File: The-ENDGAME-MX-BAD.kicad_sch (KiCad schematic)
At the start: 76 parts, among them J2 Conn_01x02_Female, SW1 SW_Push, SW10 SW_Push, SW11 SW_Push, SW12 SW_Push, SW13 SW_Push, SW14 SW_Push, SW15 SW_Push, SW16 SW_Push, SW17 SW_Push, SW18 SW_Push, SW19 SW_Push, SW2 SW_Push, SW20 SW_Push, SW21 SW_Push, SW22 SW_Push, SW23 SW_Push, SW24 SW_Push, SW25 SW_Push, SW26 SW_Push, SW27 SW_Push, SW28 SW_Push, SW29 SW_Push, SW3 SW_Push, SW30 SW_Push, SW31 SW_Push, SW32 SW_Push, SW33 SW_Push, SW34 SW_Push, SW35 SW_Push, SW36 SW_Push, SW4 SW_Push, SW5 SW_Push, SW6 SW_Push, SW7 SW_Push, SW8 SW_Push, SW9 SW_Push, U1 ProMicro-kbd-34key

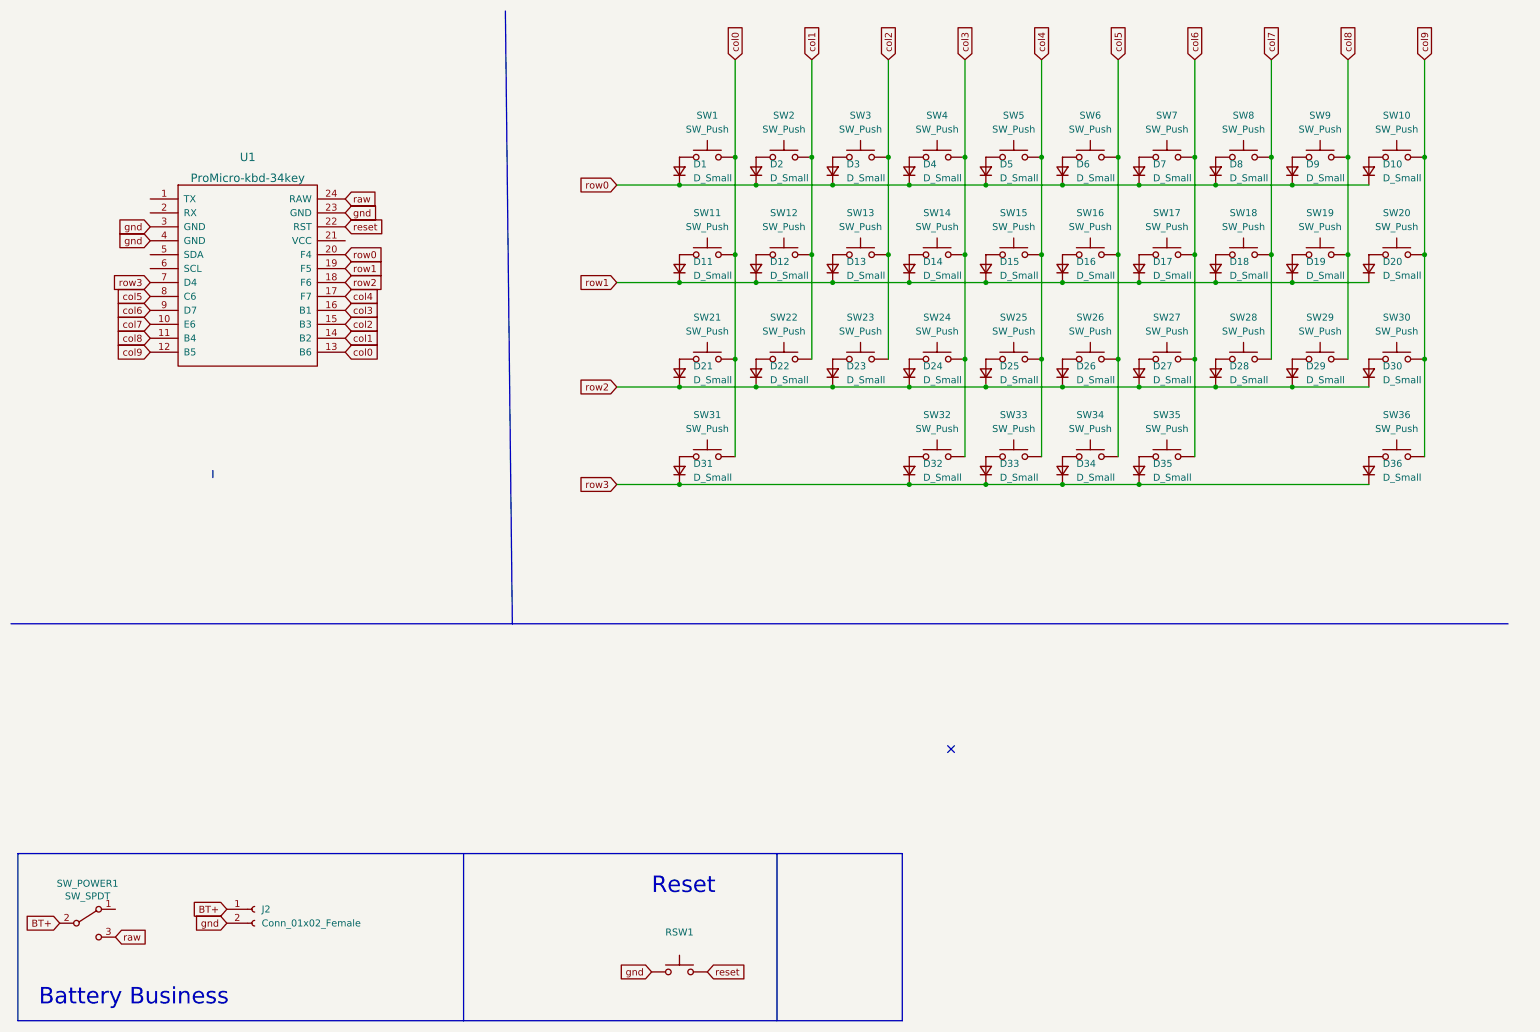
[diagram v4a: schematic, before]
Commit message: ja ja push den scheis
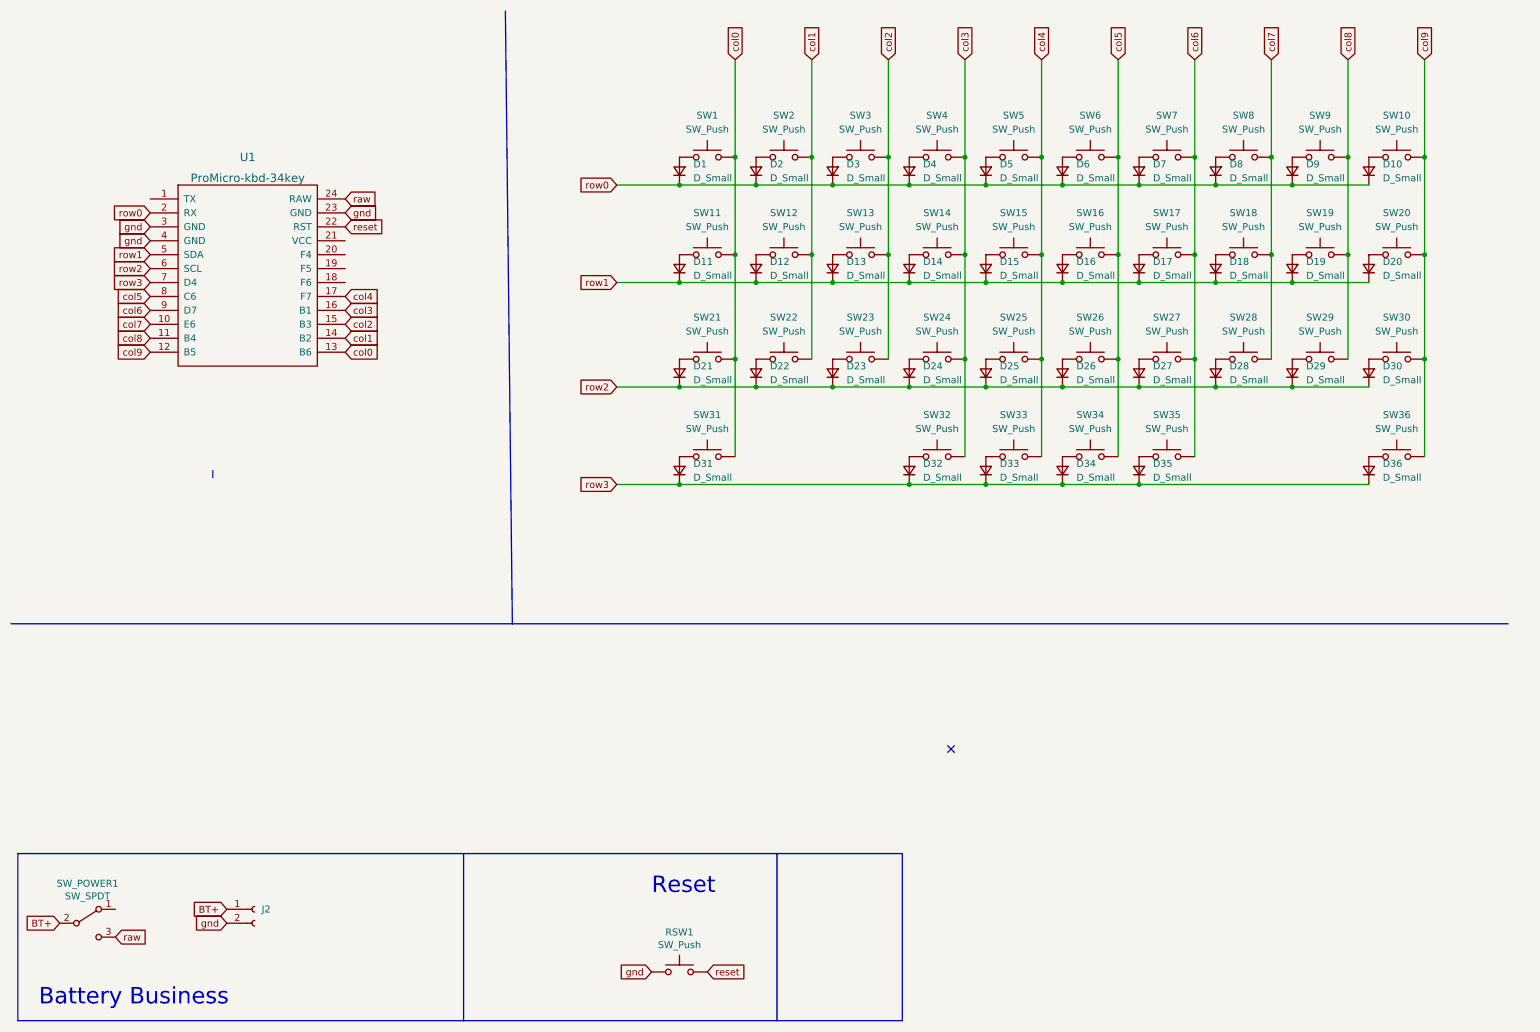
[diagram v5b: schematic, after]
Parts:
- J2: value Conn_01x02_Female -> (none); footprint Connector_JST:JST_SH_BM02B-SRSS-TB_1x02-1MP_P1.00mm_Vertical -> (none)
- RSW1: value (none) -> SW_Push; footprint (none) -> Button_Switch_SMD:SW_SPST_TL3342
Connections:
- net row0: now also U1.2 (RX); no longer U1.20 (F4)
- net row1: now also U1.5 (SDA); no longer U1.19 (F5)
- net row2: now also U1.6 (SCL); no longer U1.18 (F6)
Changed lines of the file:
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@@
     )
   )
-  (global_label "row1" (shape input) (at 73.66 59.69 0) (fields_autoplaced)
-    (effects (font (size 1.27 1.27)) (justify left))
-    (property "Intersheet References" "${INTERSHEET_REFS}" (id 0) (at 80.5483 59.7694 0)
-      (effects (font (size 1.27 1.27)) (justify left) hide)
+  (global_label "row1" (shape input) (at 38.1 57.15 180) (fields_autoplaced)
+    (effects (font (size 1.27 1.27)) (justify right))
+    (property "Intersheet References" "${INTERSHEET_REFS}" (id 0) (at 31.2117 57.0706 0)
+      (effects (font (size 1.27 1.27)) (justify right) hide)
     )
   )
@@
   (global_label "row3" (shape input) (at 38.1 62.23 180) (fields_autoplaced)
     (effects (font (size 1.27 1.27)) (justify right))
-    (property "Intersheet References" "${INTERSHEET_REFS}" (id 0) (at 31.2117 62.1506 0)
+    (property "Intersheet References" "${INTERSHEET_REFS}" (id 0) (at 31.2117 62.3094 0)
       (effects (font (size 1.27 1.27)) (justify right) hide)
     )
@@
     )
   )
-  (global_label "row2" (shape input) (at 73.66 62.23 0) (fields_autoplaced)
-    (effects (font (size 1.27 1.27)) (justify left))
-    (property "Intersheet References" "${INTERSHEET_REFS}" (id 0) (at 80.5483 62.3094 0)
-      (effects (font (size 1.27 1.27)) (justify left) hide)
+  (global_label "row2" (shape input) (at 38.1 59.69 180) (fields_autoplaced)
+    (effects (font (size 1.27 1.27)) (justify right))
+    (property "Intersheet References" "${INTERSHEET_REFS}" (id 0) (at 31.2117 59.6106 0)
+      (effects (font (size 1.27 1.27)) (justify right) hide)
     )
   )
@@
     )
   )
-  (global_label "row0" (shape input) (at 73.66 57.15 0) (fields_autoplaced)
-    (effects (font (size 1.27 1.27)) (justify left))
-    (property "Intersheet References" "${INTERSHEET_REFS}" (id 0) (at 80.5483 57.2294 0)
-      (effects (font (size 1.27 1.27)) (justify left) hide)
+  (global_label "row0" (shape input) (at 38.1 49.53 180) (fields_autoplaced)
+    (effects (font (size 1.27 1.27)) (justify right))
+    (property "Intersheet References" "${INTERSHEET_REFS}" (id 0) (at 31.2117 49.4506 0)
+      (effects (font (size 1.27 1.27)) (justify right) hide)
     )
   )
@@
     (in_bom yes) (on_board yes)
     (property "Reference" "RSW1" (id 0) (at 134.62 180.721 0))
-    (property "Value" "" (id 1) (at 134.62 183.0324 0))
-    (property "Footprint" "" (id 2) (at 134.62 182.88 0)
+    (property "Value" "SW_Push" (id 1) (at 134.62 183.0324 0))
+    (property "Footprint" "Button_Switch_SMD:SW_SPST_TL3342" (id 2) (at 134.62 182.88 0)
       (effects (font (size 1.27 1.27)) hide)
     )
@@
       (effects (font (size 1.27 1.27)) (justify left))
     )
-    (property "Value" "Conn_01x02_Female" (id 1) (at 58.42 179.0699 0)
+    (property "Value" "" (id 1) (at 58.42 179.0699 0)
       (effects (font (size 1.27 1.27)) (justify left))
     )
-    (property "Footprint" "Connector_JST:JST_SH_BM02B-SRSS-TB_1x02-1MP_P1.00mm_Vertical" (id 2) (at 57.15 176.53 0)
+    (property "Footprint" "" (id 2) (at 57.15 176.53 0)
       (effects (font (size 1.27 1.27)) hide)
     )
@@
     )
     (path "/f9b90d5e-d0d7-4775-88de-46a5d114a3f8"
-      (reference "J2") (unit 1) (value "Conn_01x02_Female") (footprint "Connector_JST:JST_SH_BM02B-SRSS-TB_1x02-1MP_P1.00mm_Vertical")
+      (reference "J2") (unit 1) (value "Conn_01x02_Female") (footprint "Connector_JST:JST_PH_S2B-PH-K_1x02_P2.00mm_Horizontal")
     )
     (path "/8c098b2f-e56b-4cd0-858f-8acf9e4a45b2"

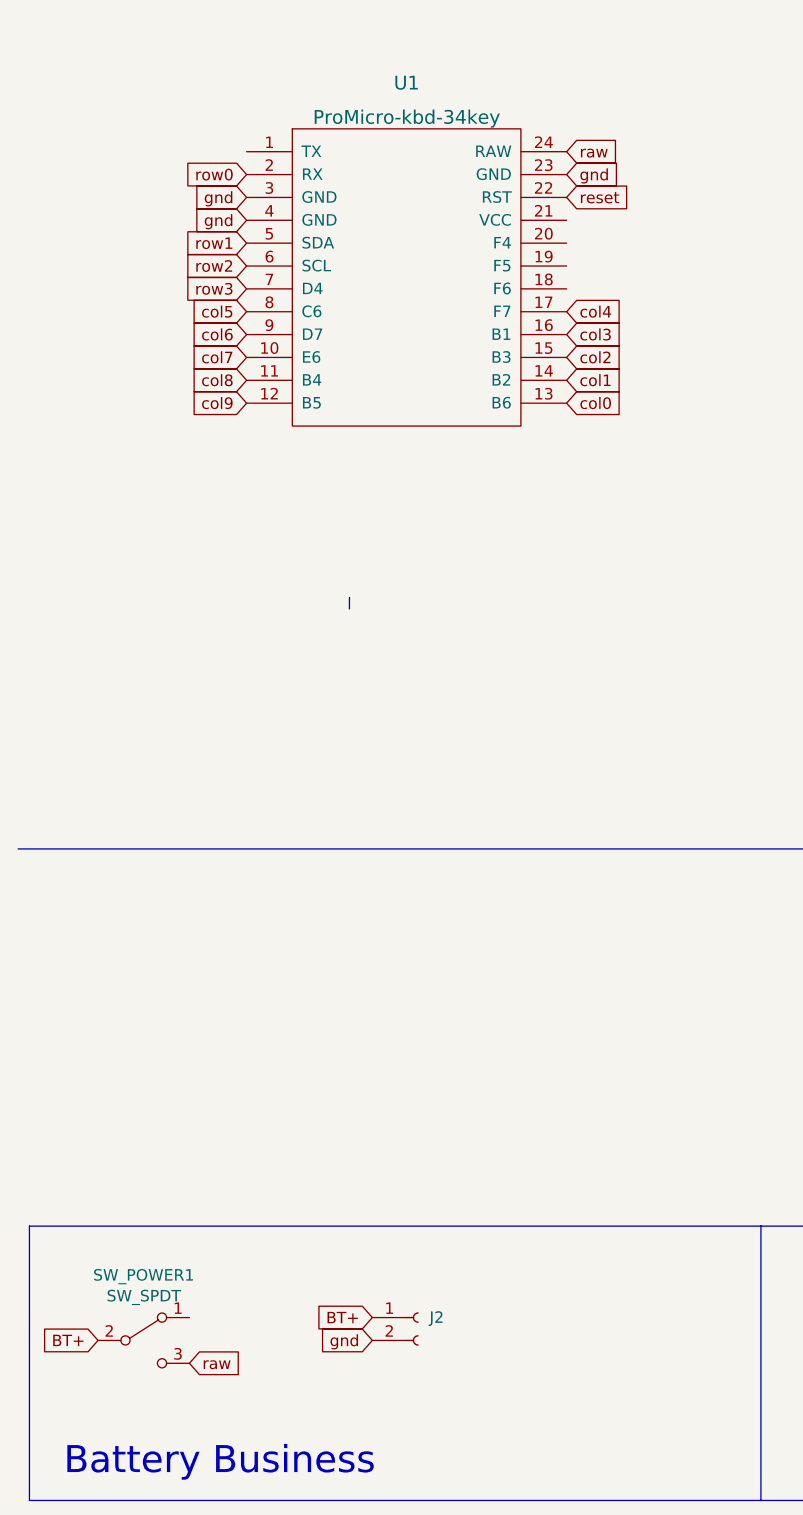
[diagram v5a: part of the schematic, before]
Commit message: back das up baby
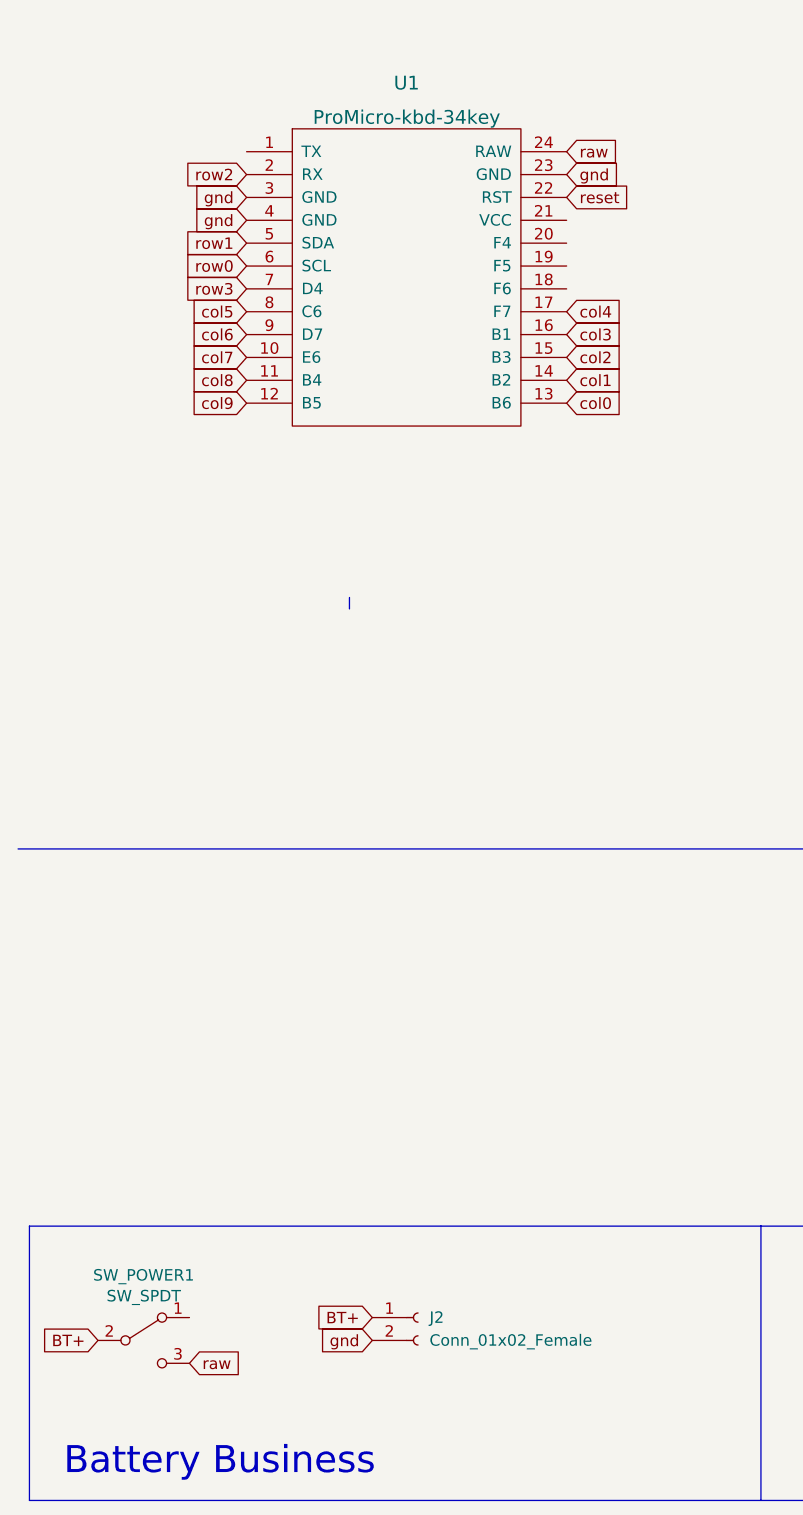
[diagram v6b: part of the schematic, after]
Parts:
- J2: value (none) -> Conn_01x02_Female; footprint (none) -> Connector_JST:JST_PH_S2B-PH-K_1x02_P2.00mm_Horizontal
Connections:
- net row0: now also U1.6 (SCL); no longer U1.2 (RX)
- net row2: now also U1.2 (RX); no longer U1.6 (SCL)
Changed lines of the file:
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@@
     )
   )
-  (global_label "row2" (shape input) (at 38.1 59.69 180) (fields_autoplaced)
+  (global_label "row2" (shape input) (at 38.1 49.53 180) (fields_autoplaced)
     (effects (font (size 1.27 1.27)) (justify right))
-    (property "Intersheet References" "${INTERSHEET_REFS}" (id 0) (at 31.2117 59.6106 0)
+    (property "Intersheet References" "${INTERSHEET_REFS}" (id 0) (at 31.2117 49.4506 0)
       (effects (font (size 1.27 1.27)) (justify right) hide)
     )
@@
     )
   )
-  (global_label "row0" (shape input) (at 38.1 49.53 180) (fields_autoplaced)
+  (global_label "row0" (shape input) (at 38.1 59.69 180) (fields_autoplaced)
     (effects (font (size 1.27 1.27)) (justify right))
-    (property "Intersheet References" "${INTERSHEET_REFS}" (id 0) (at 31.2117 49.4506 0)
+    (property "Intersheet References" "${INTERSHEET_REFS}" (id 0) (at 31.2117 59.6106 0)
       (effects (font (size 1.27 1.27)) (justify right) hide)
     )
@@
       (effects (font (size 1.27 1.27)) (justify left))
     )
-    (property "Value" "" (id 1) (at 58.42 179.0699 0)
+    (property "Value" "Conn_01x02_Female" (id 1) (at 58.42 179.0699 0)
       (effects (font (size 1.27 1.27)) (justify left))
     )
-    (property "Footprint" "" (id 2) (at 57.15 176.53 0)
-      (effects (font (size 1.27 1.27)) hide)
-    )
+    (property "Footprint" "Connector_JST:JST_PH_S2B-PH-K_1x02_P2.00mm_Horizontal" (id 2) (at 57.15 176.53 0)
+      (effects (font (size 1.27 1.27)) hide)
+    )

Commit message: biba backup
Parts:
- D1, D10, D11, D12, D13, D14, D15, D16, D17, D18, D19, D2, D20, D21, D22, D23, D24, D25, D26, D27, D28, D29, D3, D30, D31, D32, D33, D34, D35, D36, D4, D5, D6, D7, D8, D9: footprint Diode_SMD:D_SOD-123 -> (none)
- SW1, SW10, SW11, SW12, SW13, SW14, SW15, SW16, SW17, SW18, SW19, SW2, SW20, SW21, SW22, SW23, SW24, SW25, SW26, SW27, SW28, SW29, SW3, SW30, SW31, SW32, SW33, SW34, SW35, SW36, SW4, SW5, SW6, SW7, SW8, SW9: footprint keyswitches:Kailh_socket_PG1350_optional -> keyswitches:Kailh_socket_PG1350_optional_CLEAN
